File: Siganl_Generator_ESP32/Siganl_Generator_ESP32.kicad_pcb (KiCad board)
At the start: 4 copper layers, 87.6 x 107.1 mm, 45 parts, among them IC1 TPS61175QPWPRQ1, J1 Conn_01x05_Socket, J2 Conn_01x02_Socket, J3 USB_C_Receptacle_PowerOnly_6P, J4 Conn_01x19_Socket, J5 Conn_Coaxial, J6 Conn_Coaxial, SW1 SW_Push, SW2 SW_Push, SW3 SW_Push, U2 LM393

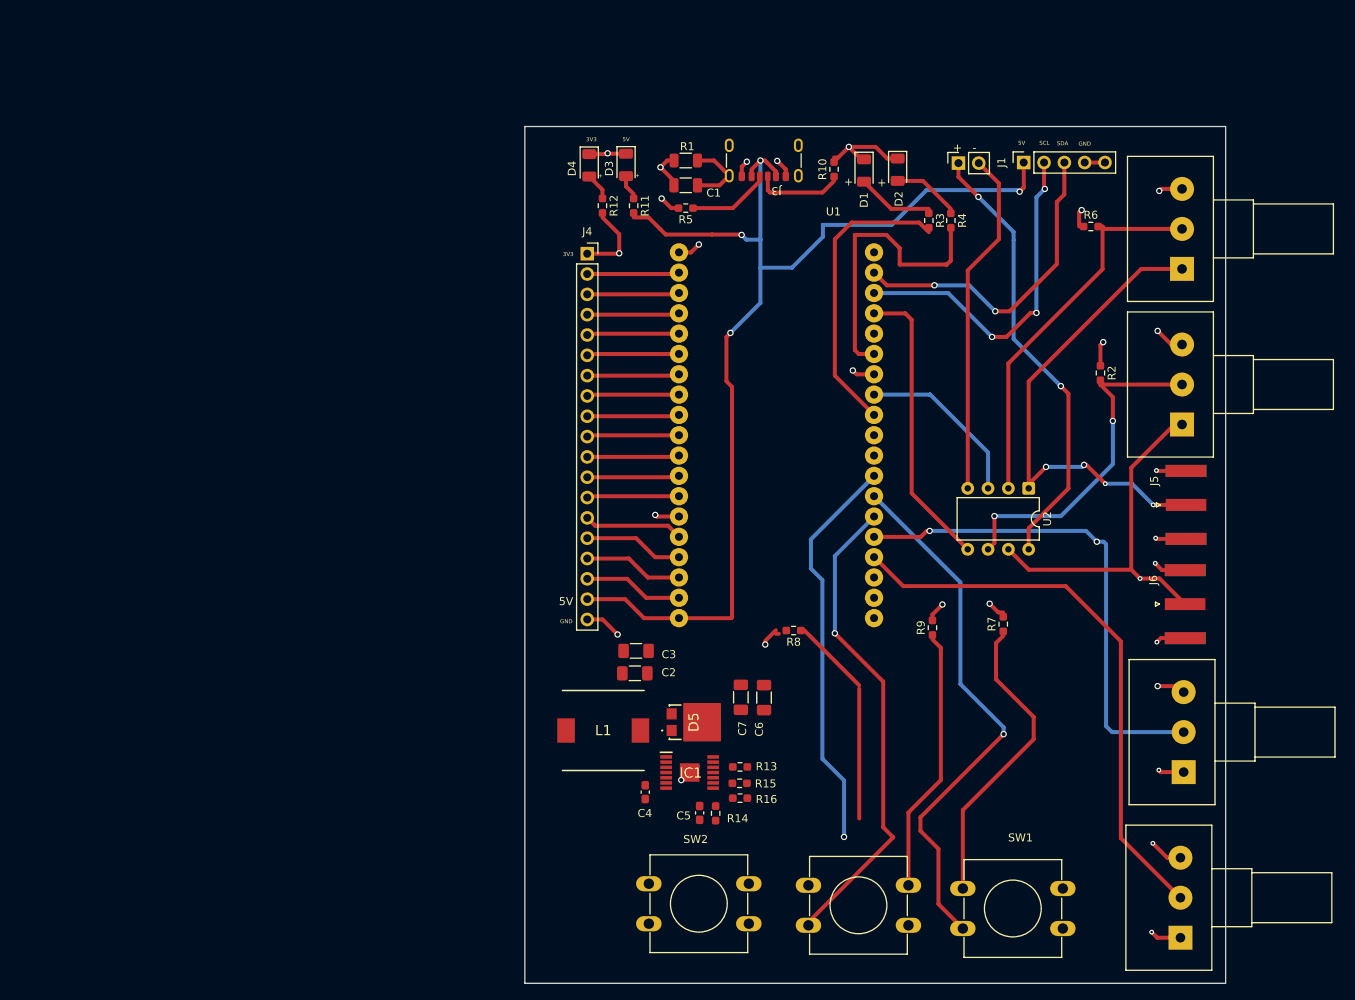
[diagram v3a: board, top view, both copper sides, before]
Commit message: new design
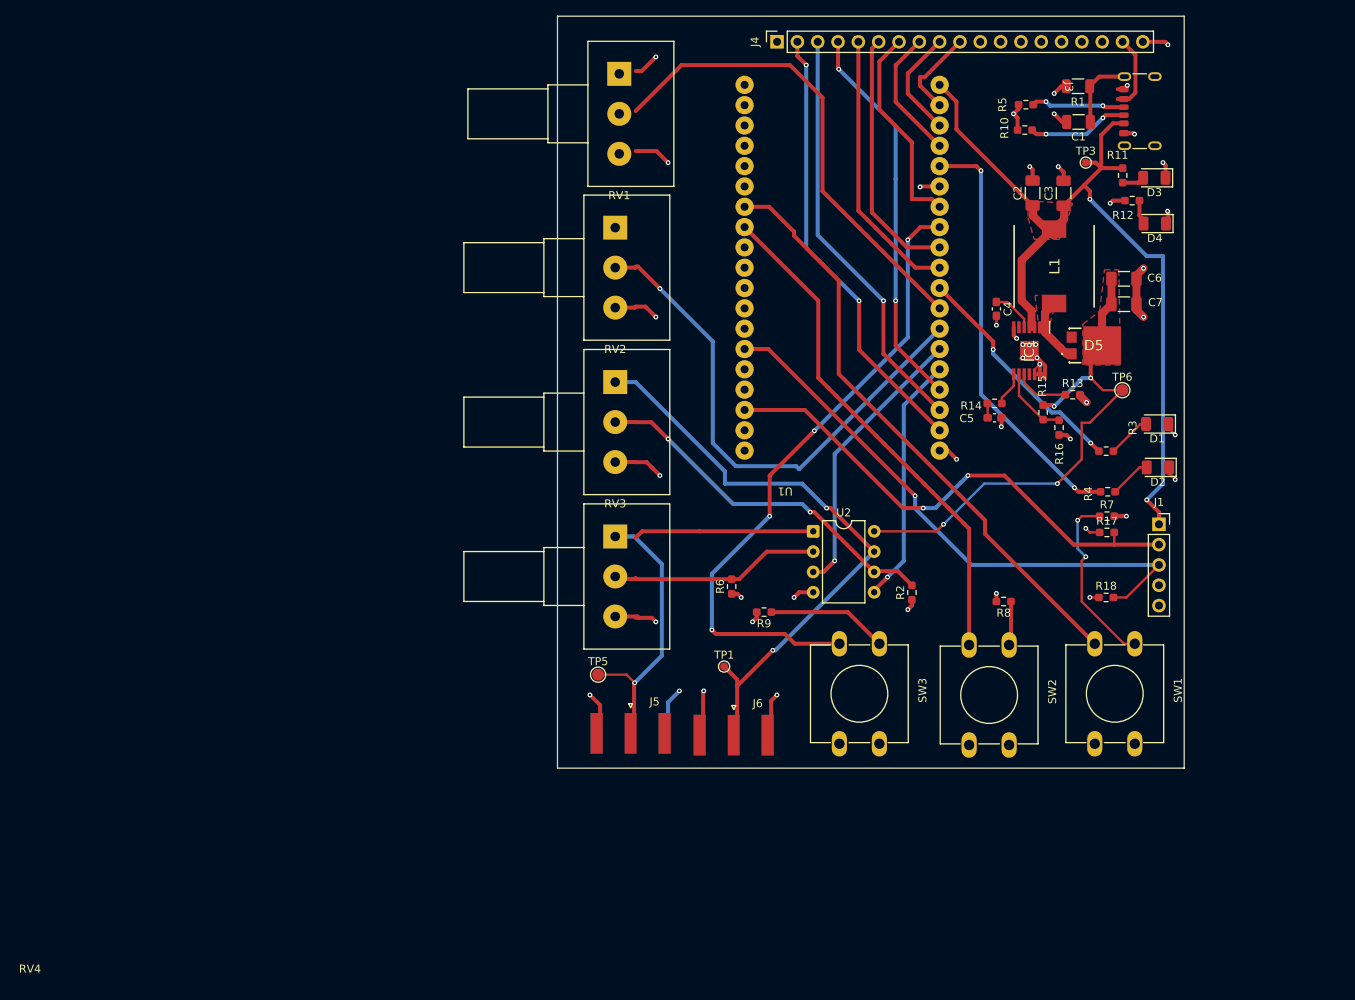
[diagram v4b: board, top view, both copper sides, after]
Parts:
- removed J2: Conn_01x02_Socket, Connector_PinSocket_2.54mm:PinSocket_1x02_P2.54mm_Vertical
- added R17: 4k7, Resistor_SMD:R_0603_1608Metric_Pad0.98x0.95mm_HandSolder, F.Cu at (127.6, 91.4)
- added R18: 4k7, Resistor_SMD:R_0603_1608Metric_Pad0.98x0.95mm_HandSolder, F.Cu at (127.5, 99.6)
- added TP1: TestPoint, TestPoint:TestPoint_Pad_D1.0mm, F.Cu at (79.8, 108.2)
- added TP3: TestPoint, TestPoint:TestPoint_Pad_D1.0mm, F.Cu at (125.0, 45.2)
- added TP5: TestPoint, TestPoint:TestPoint_Pad_D1.5mm, F.Cu at (64.0, 109.2)
- added TP6: TestPoint, TestPoint:TestPoint_Pad_D1.5mm, F.Cu at (129.5, 73.7)
- moved RV1 128.8 mm to (66.7, 34.1), turned to 0 degrees
- moved RV2 98.4 mm to (66.1, 53.3), turned to 0 degrees
- moved L1 80.9 mm to (121.0, 58.2), turned to -90 degrees
- moved RV4 78.4 mm to (66.1, 91.9), turned to 0 degrees
- moved C3 78.3 mm to (122.2, 49.0), turned to 90 degrees
- moved C2 77.9 mm to (118.3, 49.0), turned to 90 degrees
- moved J5 75.1 mm to (68.1, 116.6), turned to -90 degrees
- moved C4 74.7 mm to (113.8, 63.5)
- moved D4 71.1 mm to (133.6, 52.8), turned to 180 degrees
- moved RV3 71.1 mm to (66.1, 72.6), turned to 0 degrees
- moved C6 69.0 mm to (129.7, 59.7), turned to 0 degrees
- moved D5 68.7 mm to (126.0, 68.1)
- moved C7 68.6 mm to (129.7, 62.9), turned to 0 degrees
- moved IC1 67.7 mm to (117.9, 68.7), turned to -90 degrees
- moved R12 66.2 mm to (130.8, 50.0), turned to 180 degrees
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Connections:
- J4 pad 11: Net-(J4-Pin_11) -> unconnected-(J4-Pin_11-Pad11)
- J4 pad 12: Net-(J4-Pin_12) -> unconnected-(J4-Pin_12-Pad12)
- J4 pad 13: Net-(J4-Pin_13) -> unconnected-(J4-Pin_13-Pad13)
- J4 pad 14: Net-(J4-Pin_14) -> unconnected-(J4-Pin_14-Pad14)
- J4 pad 15: Net-(J4-Pin_15) -> unconnected-(J4-Pin_15-Pad15)
- J4 pad 16: Net-(J4-Pin_16) -> unconnected-(J4-Pin_16-Pad16)
- J4 pad 17: Net-(J4-Pin_17) -> unconnected-(J4-Pin_17-Pad17)
- U1 pad 10: Net-(J4-Pin_10) -> Net-(J4-Pin_5)
- U1 pad 11: Net-(J4-Pin_11) -> Net-(J4-Pin_6)
- U1 pad 12: Net-(J4-Pin_12) -> Buttom 3
- U1 pad 13: Net-(J4-Pin_13) -> Net-(J4-Pin_7)
- U1 pad 15: Net-(J4-Pin_14) -> LED_Green
- U1 pad 16: Net-(J4-Pin_15) -> Net-(J4-Pin_8)
- U1 pad 17: Net-(J4-Pin_16) -> Net-(J4-Pin_9)
- U1 pad 18: Net-(J4-Pin_17) -> Net-(J4-Pin_10)
- U1 pad 21: OLED_SDA -> unconnected-(U1-G23-Pad21)
- U1 pad 23: Signal 1 -> unconnected-(U1-TDX-Pad23)
- U1 pad 25: LED_Green -> OLED_SDA
- U1 pad 27: Signal 2 -> unconnected-(U1-G19-Pad27)
- U1 pad 28: Led_Red -> unconnected-(U1-G18-Pad28)
- U1 pad 33: Buttom 3 -> unconnected-(U1-G0-Pad33)
- U1 pad 34: G34 Frquenz -> unconnected-(U1-G2-Pad34)
- U1 pad 35: G35 DutyCycle -> unconnected-(U1-G15-Pad35)
- U1 pad 5: Net-(J4-Pin_5) -> Signal 1
- U1 pad 6: Net-(J4-Pin_6) -> Signal 2
- U1 pad 7: Net-(J4-Pin_7) -> G34 Frquenz
- U1 pad 8: Net-(J4-Pin_8) -> G35 DutyCycle
- U1 pad 9: Net-(J4-Pin_9) -> Led_Red
- U2 pad 4: -12 V -> GND
- U2 pad 8: 12 V -> 25V
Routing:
- net 25V: track 0.00 -> 66.6 mm, vias 0 -> 4
- net 12 V: track 56.0 -> 0.00 mm, vias 2 -> 0
- net Net-(J4-Pin_2): track 11.6 -> 55.9 mm, vias 0 -> 2
- net -12 V: track 43.3 -> 0.00 mm
- net Net-(J4-Pin_3): track 11.6 -> 52.3 mm, vias 0 -> 1
- net Net-(J4-Pin_4): track 11.6 -> 48.7 mm, vias 0 -> 2
- net OLED_SDA: track 40.3 -> 71.3 mm, vias 2 -> 1
- net Signal 1 Output: track 46.3 -> 74.1 mm, vias 1 -> 2
- net Net-(J4-Pin_5): track 11.6 -> 34.2 mm
- net 5 V: track 142.1 -> 120.2 mm, vias 4 -> 2
- net Net-(U2A--): track 47.7 -> 26.5 mm
- net OLED_SCL: track 43.1 -> 63.7 mm, vias 3 -> 2
- net Net-(R8-Pad1): track 26.0 -> 5.53 mm
- net Net-(J4-Pin_6): track 11.6 -> 32.0 mm
- net Buttom 3: track 60.6 -> 80.6 mm, vias 1 -> 4
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- added copper zone on F.Cu, net (none)
- added copper zone on F.Cu, net 25V
- added copper zone on F.Cu, net 5 V
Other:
- board size 87.6 x 107.1 mm -> 78.3 x 94 mm
- board text removed: "+"
- board text removed: "-"
- board text removed: "GND"
- board text removed: "SCL"
- board text removed: "SDA"
- board text removed: "Siganl Gererater v.1 designed by Amjad Trablsi"
